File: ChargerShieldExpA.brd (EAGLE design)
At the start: 161.3 x 99.1 mm, 101 parts, among them IC1 TL431, IC2 LM324N, Q1 BUZ11, Q2 BD648, Q3 BUZ171, Q4 IRFZ48Z, T1 BC548, X1 +Vin, X2 VCC, X3 Battery

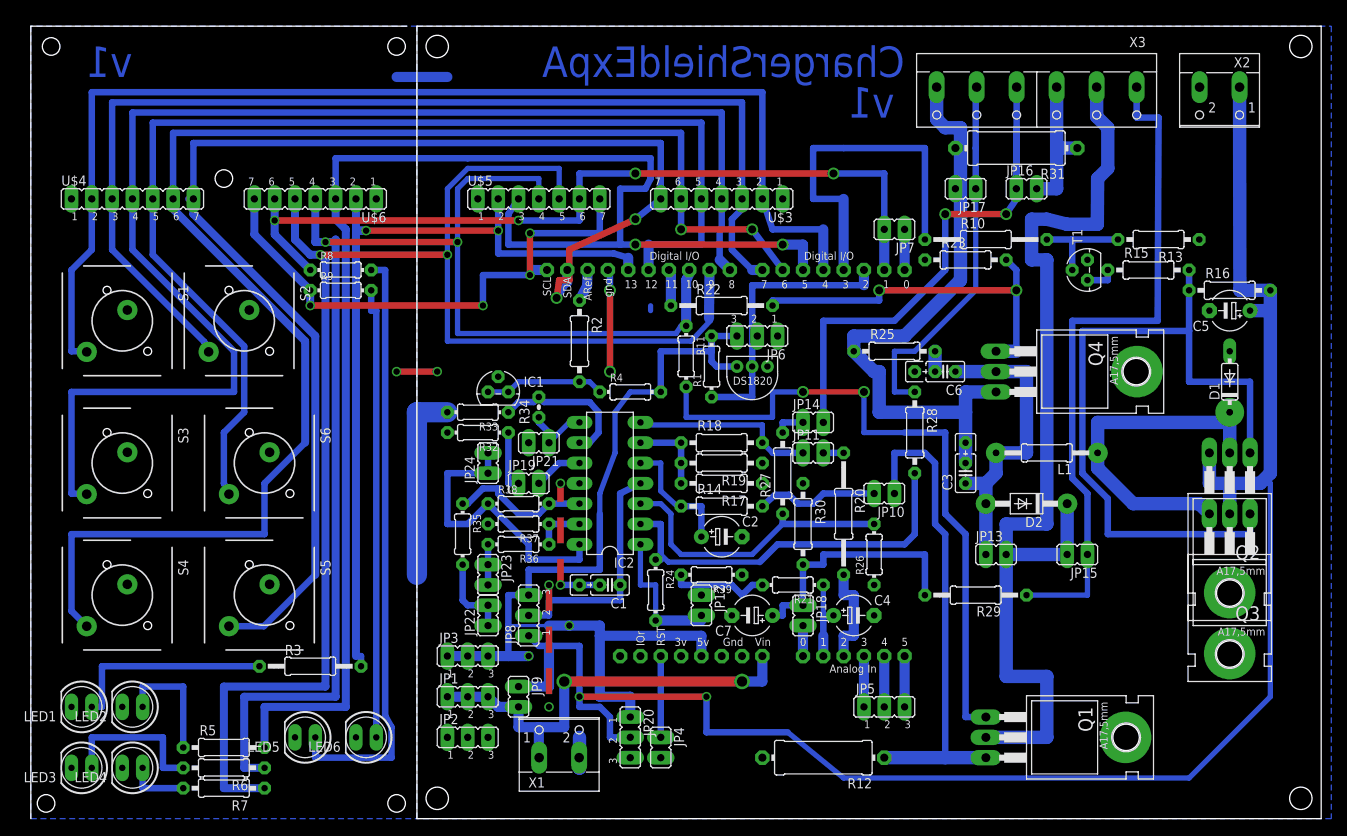
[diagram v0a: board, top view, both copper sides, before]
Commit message: Production version v1
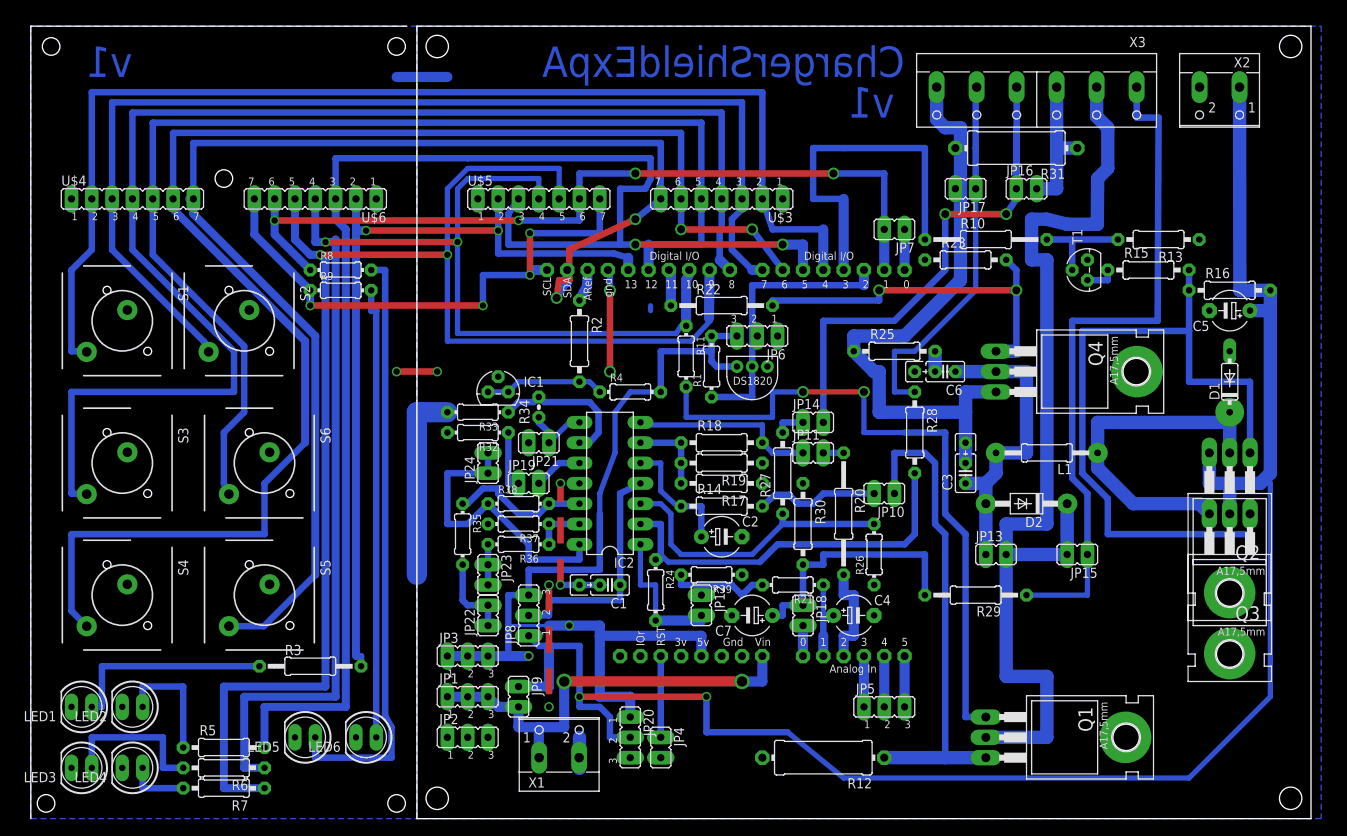
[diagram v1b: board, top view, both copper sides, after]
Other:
- board size 161.3 x 99.1 mm -> 160 x 99.1 mm
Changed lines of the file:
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@@
 <setting verticaltext="up"/>
 </settings>
-<grid distance="0.05" unitdist="inch" unit="mm" style="lines" multiple="1" display="yes" altdistance="0.025" altunitdist="inch" altunit="mm"/>
+<grid distance="2.54" unitdist="mm" unit="mm" style="lines" multiple="1" display="yes" altdistance="1.27" altunitdist="mm" altunit="mm"/>
 <layers>
-<layer number="1" name="Top" color="4" fill="1" visible="yes" active="yes"/>
+<layer number="1" name="Top" color="4" fill="1" visible="no" active="yes"/>
 <layer number="2" name="Route2" color="1" fill="3" visible="no" active="no"/>
 <layer number="3" name="Route3" color="4" fill="3" visible="no" active="no"/>
@@
 <layer number="17" name="Pads" color="2" fill="1" visible="yes" active="yes"/>
 <layer number="18" name="Vias" color="2" fill="1" visible="yes" active="yes"/>
-<layer number="19" name="Unrouted" color="6" fill="1" visible="yes" active="yes"/>
+<layer number="19" name="Unrouted" color="6" fill="1" visible="no" active="yes"/>
 <layer number="20" name="Dimension" color="15" fill="1" visible="yes" active="yes"/>
-<layer number="21" name="tPlace" color="7" fill="1" visible="yes" active="yes"/>
-<layer number="22" name="bPlace" color="7" fill="1" visible="yes" active="yes"/>
-<layer number="23" name="tOrigins" color="15" fill="1" visible="yes" active="yes"/>
-<layer number="24" name="bOrigins" color="15" fill="1" visible="yes" active="yes"/>
-<layer number="25" name="tNames" color="7" fill="1" visible="yes" active="yes"/>
+<layer number="21" name="tPlace" color="7" fill="1" visible="no" active="yes"/>
+<layer number="22" name="bPlace" color="7" fill="1" visible="no" active="yes"/>
+<layer number="23" name="tOrigins" color="15" fill="1" visible="no" active="yes"/>
+<layer number="24" name="bOrigins" color="15" fill="1" visible="no" active="yes"/>
+<layer number="25" name="tNames" color="7" fill="1" visible="no" active="yes"/>
 <layer number="26" name="bNames" color="7" fill="1" visible="no" active="yes"/>
 <layer number="27" name="tValues" color="7" fill="1" visible="no" active="yes"/>
@@
 <layer number="43" name="vRestrict" color="2" fill="10" visible="no" active="yes"/>
 <layer number="44" name="Drills" color="7" fill="1" visible="no" active="yes"/>
-<layer number="45" name="Holes" color="7" fill="1" visible="yes" active="yes"/>
+<layer number="45" name="Holes" color="7" fill="1" visible="no" active="yes"/>
 <layer number="46" name="Milling" color="3" fill="1" visible="no" active="yes"/>
 <layer number="47" name="Measures" color="7" fill="1" visible="no" active="yes"/>
@@
 <layer number="49" name="Reference" color="7" fill="1" visible="no" active="yes"/>
 <layer number="50" name="dxf" color="7" fill="1" visible="no" active="no"/>
-<layer number="51" name="tDocu" color="7" fill="1" visible="yes" active="yes"/>
+<layer number="51" name="tDocu" color="7" fill="1" visible="no" active="yes"/>
 <layer number="52" name="bDocu" color="7" fill="1" visible="no" active="yes"/>
 <layer number="53" name="tGND_GNDA" color="7" fill="9" visible="no" active="no"/>
@@
 <layer number="112" name="tSilk" color="7" fill="1" visible="no" active="yes"/>
 <layer number="113" name="IDFDebug" color="4" fill="1" visible="no" active="yes"/>
-<layer number="116" name="centerDrill" color="9" fill="4" visible="no" active="yes"/>
+<layer number="116" name="centerDrill" color="9" fill="4" visible="yes" active="yes"/>
 <layer number="121" name="_tsilk" color="7" fill="1" visible="no" active="yes"/>
 <layer number="122" name="_bsilk" color="7" fill="1" visible="no" active="yes"/>
@@
 <board>
 <plain>
-<wire x1="2.54" y1="81.28" x2="115.57" y2="81.28" width="0.1" layer="20"/>
-<wire x1="115.57" y1="81.28" x2="115.57" y2="-17.78" width="0.1" layer="20"/>
-<wire x1="115.57" y1="-17.78" x2="2.54" y2="-17.78" width="0.1" layer="20"/>
+<wire x1="2.54" y1="81.28" x2="114.3" y2="81.28" width="0.1" layer="20"/>
+<wire x1="114.3" y1="81.28" x2="114.3" y2="-17.78" width="0.1" layer="20"/>
+<wire x1="114.3" y1="-17.78" x2="2.54" y2="-17.78" width="0.1" layer="20"/>
 <wire x1="2.54" y1="-17.78" x2="2.54" y2="81.28" width="0.1" layer="20"/>
 <hole x="5.08" y="-15.24" drill="2.8"/>
 <hole x="5.08" y="78.74" drill="2.8"/>
-<hole x="113.03" y="-15.24" drill="2.8"/>
-<hole x="113.03" y="78.74" drill="2.8"/>
+<hole x="111.76" y="-15.24" drill="2.8"/>
+<hole x="111.76" y="78.74" drill="2.8"/>
 <wire x1="-45.72" y1="-17.78" x2="-45.72" y2="81.28" width="0.1" layer="20"/>
 <wire x1="-45.72" y1="81.28" x2="1.27" y2="81.28" width="0.1" layer="20"/>
@@
 <circle x="5.08" y="-15.24" radius="0.9" width="1.1" layer="116"/>
 <circle x="5.08" y="78.74" radius="0.9" width="1.1" layer="116"/>
-<circle x="113.03" y="-15.24" radius="0.9" width="1.1" layer="116"/>
-<circle x="113.03" y="78.74" radius="0.9" width="1.1" layer="116"/>
+<circle x="111.76" y="-15.24" radius="0.9" width="1.1" layer="116"/>
+<circle x="111.76" y="78.74" radius="0.9" width="1.1" layer="116"/>
 <circle x="-43.18" y="78.74" radius="0.75" width="0.8" layer="116"/>
 <circle x="0" y="78.74" radius="0.75" width="0.8" layer="116"/>
@@
 <circle x="-2.54" y="-7.62" radius="0.4" width="0.1" layer="116"/>
 <circle x="-5.08" y="-7.62" radius="0.4" width="0.1" layer="116"/>
+<circle x="91.186" y="-7.62" radius="1.026" width="1.351" layer="116"/>
 <circle x="73.66" y="-5.08" radius="0.479" width="0.259" layer="116"/>
 <circle x="73.66" y="-7.62" radius="0.479" width="0.259" layer="116"/>
 <circle x="73.66" y="-10.16" radius="0.479" width="0.259" layer="116"/>
+<circle x="104.14" y="10.414" radius="1.025" width="1.351" layer="116"/>
 <circle x="106.68" y="27.94" radius="0.479" width="0.259" layer="116"/>
 <circle x="104.14" y="27.94" radius="0.479" width="0.259" layer="116"/>
 <circle x="101.6" y="27.94" radius="0.479" width="0.259" layer="116"/>
+<circle x="104.14" y="2.794" radius="1.025" width="1.351" layer="116"/>
 <circle x="106.68" y="20.32" radius="0.479" width="0.259" layer="116"/>
 <circle x="104.14" y="20.32" radius="0.479" width="0.259" layer="116"/>
 <circle x="101.6" y="20.32" radius="0.479" width="0.259" layer="116"/>
+<circle x="92.456" y="38.1" radius="1.025" width="1.351" layer="116"/>
 <circle x="74.93" y="38.1" radius="0.479" width="0.259" layer="116"/>
 <circle x="74.93" y="40.64" radius="0.479" width="0.259" layer="116"/>
@@
 <circle x="68.58" y="57.785" radius="0.45" width="0.2" layer="116"/>
 <circle x="76.2" y="57.785" radius="0.45" width="0.2" layer="116"/>
+<circle x="92.551" y="38.1" radius="0.4" width="0.1" layer="116"/>
+<circle x="104.14" y="10.478" radius="0.4" width="0.1" layer="116"/>
+<circle x="104.14" y="2.857" radius="0.4" width="0.1" layer="116"/>
+<circle x="91.123" y="-7.62" radius="0.4" width="0.1" layer="116"/>
+<circle x="74.93" y="27.94" radius="0.4" width="0.1" layer="116"/>
+<circle x="87.63" y="27.94" radius="0.4" width="0.1" layer="116"/>
+<circle x="73.66" y="21.59" radius="0.4" width="0.1" layer="116"/>
+<circle x="83.82" y="21.59" radius="0.4" width="0.1" layer="116"/>
+<circle x="104.14" y="33.02" radius="0.4" width="0.1" layer="116"/>
 <circle x="-8.89" y="54.293" radius="0.4" width="0.1" layer="116"/>
 <circle x="7.62" y="54.293" radius="0.4" width="0.1" layer="116"/>
@@
 <vertex x="2.54" y="-17.78"/>
 <vertex x="2.54" y="81.28"/>
-<vertex x="116.84" y="81.28"/>
-<vertex x="116.84" y="-17.78"/>
+<vertex x="115.57" y="81.28"/>
+<vertex x="115.57" y="-17.78"/>
 </polygon>
 <contactref element="R13" pad="1"/>

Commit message: rearranged, better DRC
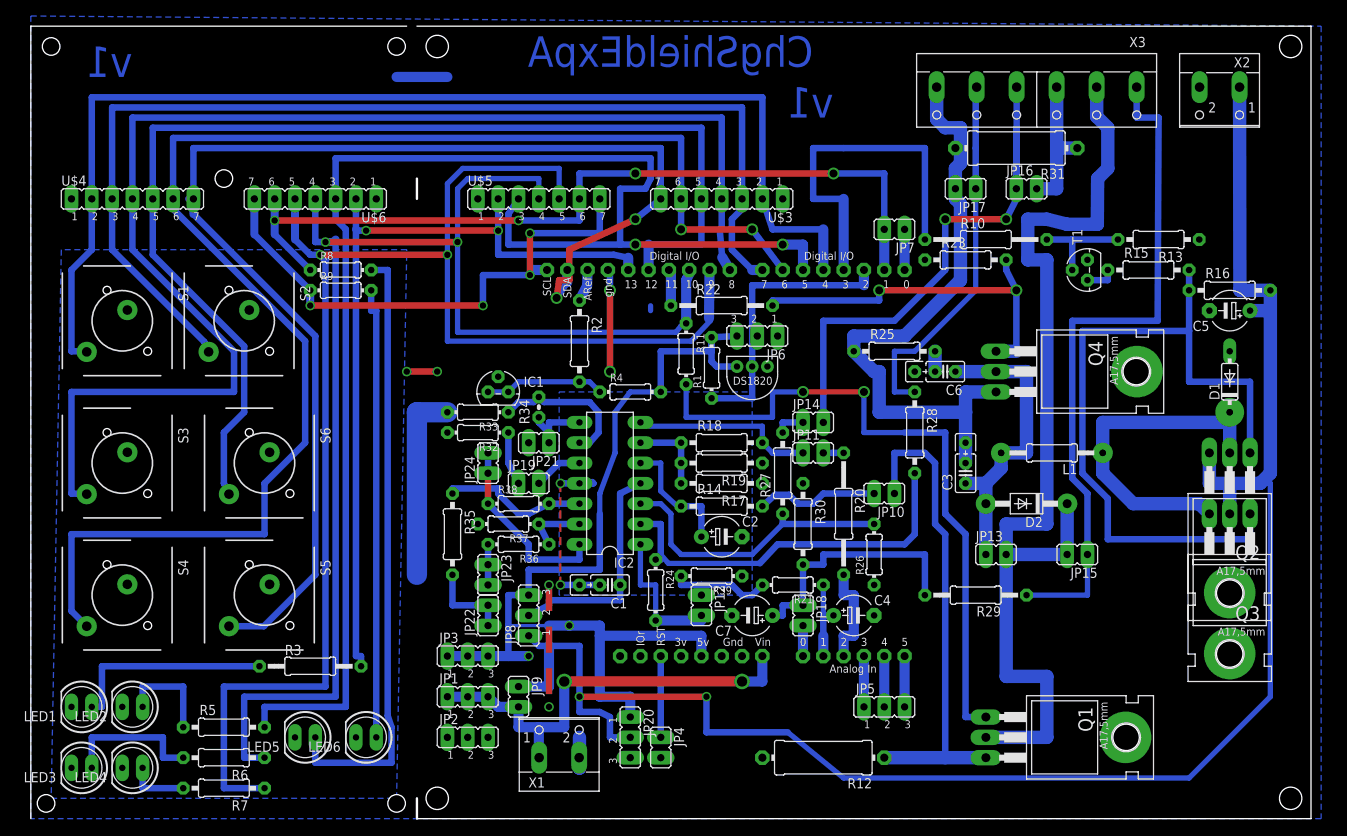
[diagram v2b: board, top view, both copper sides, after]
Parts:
- R35: device rcl:0204/7 -> rcl:0207/10
- moved R5 2.54 mm to (-21.6, -6.35)
- moved R35 1.27 mm to (6.99, 17.8)
- moved R37 1.27 mm to (14.0, 19.1)
- moved R6 1.27 mm to (-21.6, -10.2)
- moved L1 0.64 mm to (81.9, 27.9)
- moved R11 0.32 mm to (36.2, 40.3)
- moved R39 0.16 mm to (39.4, 12.5)
- moved R1 0.16 mm to (39.4, 38.6)
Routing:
- net N$48: track 37.4 -> 23.7 mm
- net GND: track 164.6 -> 168.7 mm
- net N$24: track 15.2 -> 12.7 mm
- net N$19: track 183.9 -> 181.4 mm
- net PWM_DISCHARGE1: track 172.4 -> 170.6 mm
- net N$36: track 6.35 -> 7.92 mm
- net N$31: track 169.2 -> 167.7 mm
- net N$34: track 8.56 -> 10.1 mm
- net N$39: track 75.0 -> 76.4 mm
- net N$26: track 148.0 -> 146.7 mm
- net N$23: track 146.2 -> 144.9 mm
- net N$20: track 19.0 -> 17.8 mm
- net N$7: track 90.9 -> 92.1 mm
- net N$38: track 164.2 -> 162.9 mm
- net N$37: track 186.3 -> 185.1 mm
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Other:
- outline, holes or cut-outs redrawn
- board text added: "ChgShieldExpA"
- board text removed: "ChargerShieldExpA"
